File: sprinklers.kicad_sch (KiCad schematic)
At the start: 43 parts, among them J1 Conn_01x02, J2 Conn_01x02, J3 Conn_01x02, J4 Conn_01x02, J5 Conn_01x02, J6 Conn_01x02, K1 SANYOU_SRD_Form_C, K2 SANYOU_SRD_Form_C, K3 SANYOU_SRD_Form_C, K4 SANYOU_SRD_Form_C, K5 SANYOU_SRD_Form_C, K6 SANYOU_SRD_Form_C, Q1 Q_NMOS_GDS, Q2 Q_NMOS_GDS, Q3 Q_NMOS_GDS, Q4 Q_NMOS_GDS, Q5 Q_NMOS_GDS, Q6 Q_NMOS_GDS, U1 LM2596S-5, U2 ESP32-WROOM-32D, U3 AP1117-33

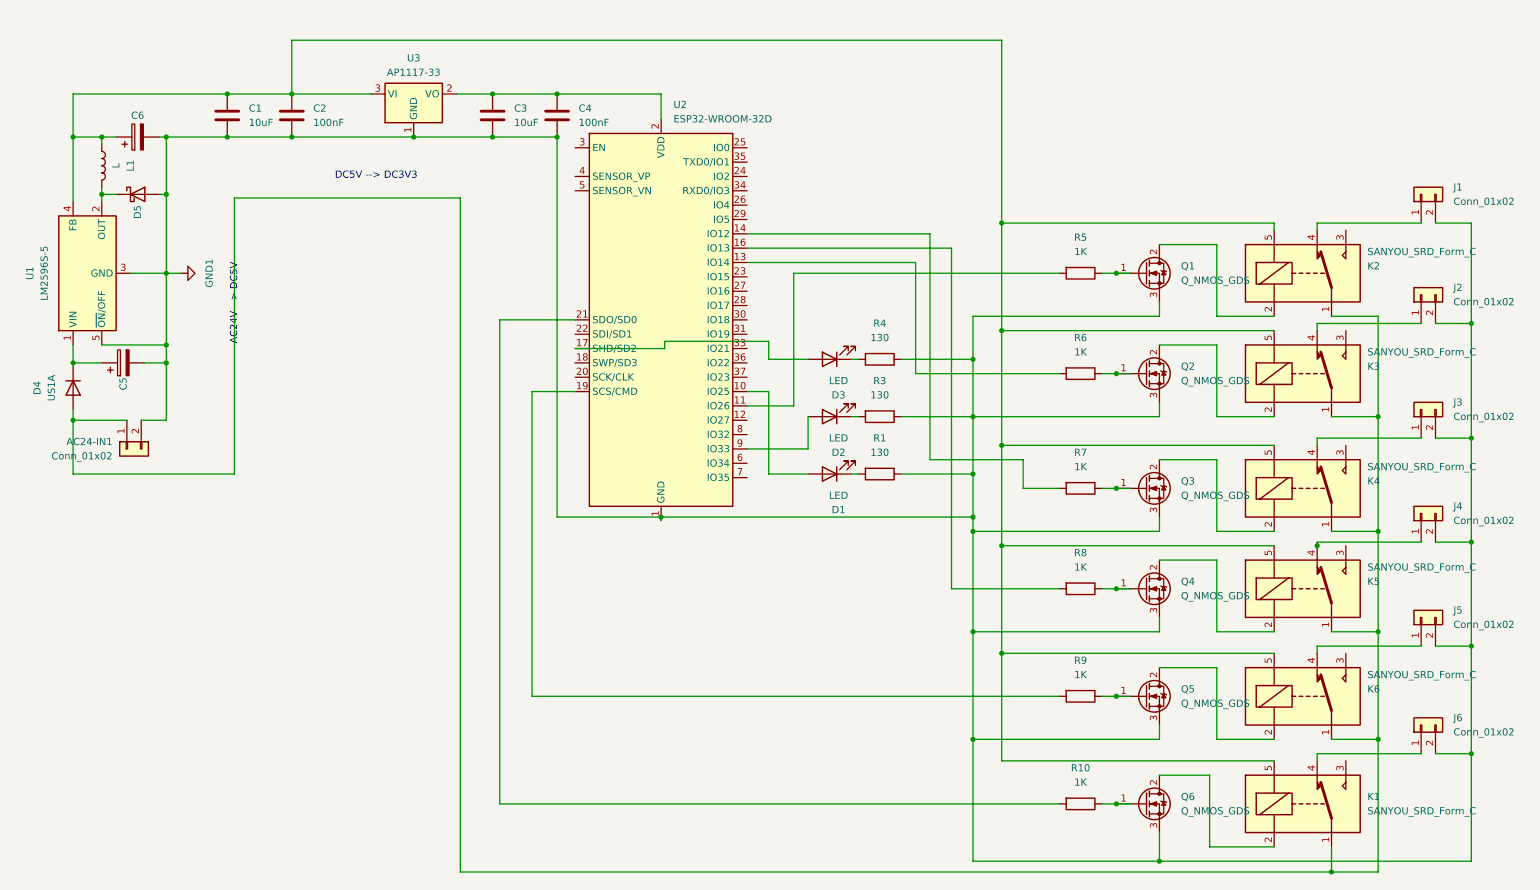
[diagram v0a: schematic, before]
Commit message: V1.1.0 with notation
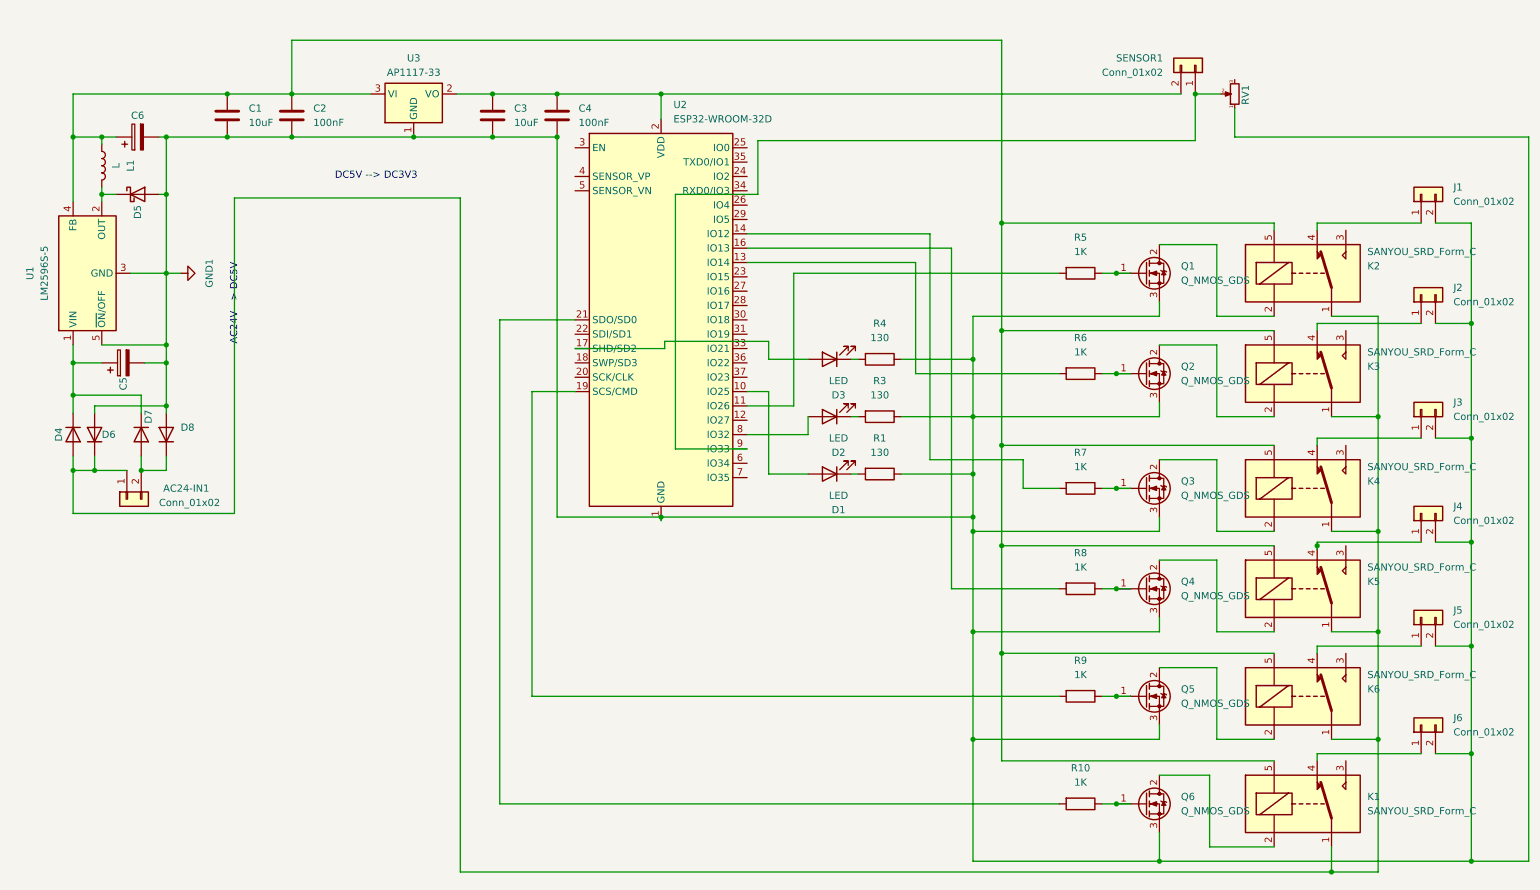
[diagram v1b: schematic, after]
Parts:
- added D6, D7, D8: 900mV@2A 30ns 2A 50V DO-214AA Diodes, Diode_SMD:D_SMB, symbol Diode:US1A
- added RV1: R_Potentiometer_Small, Potentiometer_THT:Potentiometer_Bourns_3296Y_Vertical, symbol Device:R_Potentiometer_Small
- added SENSOR1: Conn_01x02, Connector:JWT_A3963_1x02_P3.96mm_Vertical, symbol Connector_Generic:Conn_01x02
- AC24-IN1, J1, J2, J3, J4, J5, J6: LCSC C474894 -> C3031444
- C1: footprint Capacitor_SMD:C_0402_1005Metric -> Capacitor_SMD:C_0805_2012Metric
- C2, C4: footprint Capacitor_SMD:C_0402_1005Metric -> Capacitor_SMD:C_0603_1608Metric
- C3: footprint Capacitor_SMD:C_0402_1005Metric -> Capacitor_SMD:C_0805_2012Metric; LCSC C13585 -> C440198
- D1: LCSC C2297 -> C84256
- D2: LCSC C2296 -> C2297
- D3: LCSC C84256 -> C2296
- D4: value US1A -> 900mV@2A 30ns 2A 50V DO-214AA Diodes; footprint Diode_SMD:D_SMA -> Diode_SMD:D_SMB; LCSC C183422 -> C5224093
- Q1, Q2, Q3, Q4, Q5, Q6: LCSC C98152 -> C122491
- R9: LCSC C17451 -> C4410
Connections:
- net GND1: now also D6.2 (A), D8.2 (A), RV1.1; no longer AC24-IN1.2 (Pin_2)
- net at AC24-IN1.1 (Pin_1), D4.2 (A), K1.1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: now also D6.1 (K)
- net at C3.1, C4.1, U2.2 (VDD)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: now also SENSOR1.2 (Pin_2)
- net at C5.1, D4.1 (K), U1.1 (VIN): now also D7.1 (K)
- net at U2.9 (IO33): now also RV1.2, SENSOR1.1 (Pin_1); no longer D2.2 (A)
- net at U2.8 (IO32): now also D2.2 (A)
- new net: AC24-IN1.2 (Pin_2), D7.2 (A), D8.1 (K)
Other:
- moved on the sheet: AC24-IN1, D4

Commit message: applying fixed after review
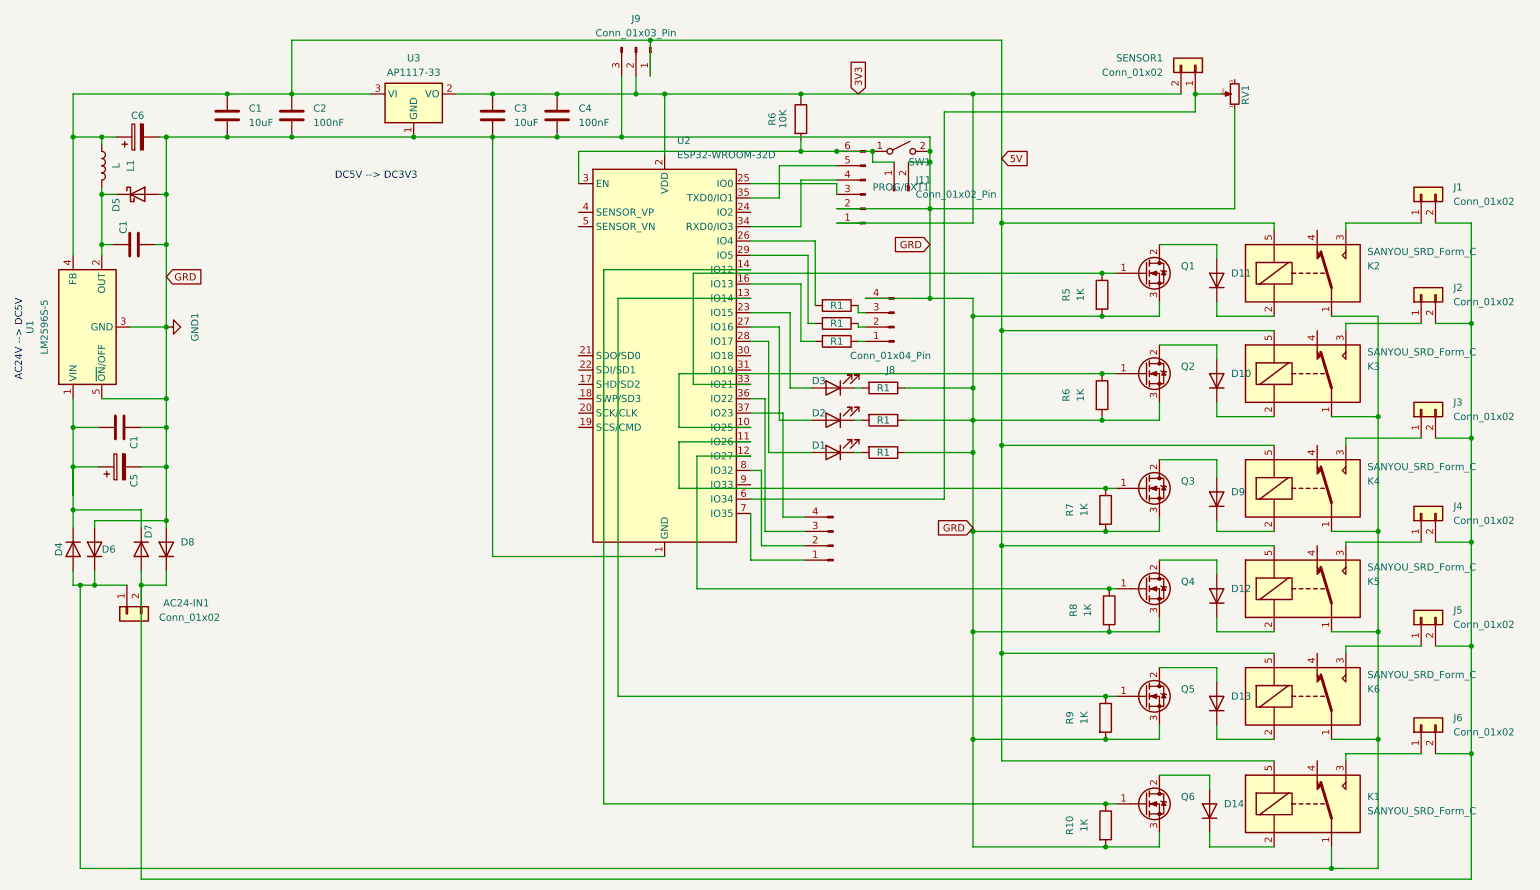
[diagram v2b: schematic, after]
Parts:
- removed R3, R4: 130, Resistor_SMD:R_1206_3216Metric, symbol Device:R
- removed R6: 1K, Resistor_SMD:R_1206_3216Metric, symbol Device:R
- added C1 (x2): 25V 1uF X5R ±10% 0402 Multilayer Ceramic Capacito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, Capacitor_SMD:C_01005_0402Metric, symbol Device:C
- added D10, D11, D12, D13, D14, D9: 75V 400mW Single 1V@50mA 4ns 150mA SOD-123 Switch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, Diode_SMD:D_SOD-123, symbol Diode:US1A
- added EXT1, J8: Conn_01x04_Pin, Connector_PinHeader_2.54mm:PinHeader_1x04_P2.54mm_Vertical, symbol Connector:Conn_01x04_Pin
- added J11: Conn_01x02_Pin, Connector_PinHeader_2.54mm:PinHeader_1x02_P2.54mm_Vertical, symbol Connector:Conn_01x02_Pin
- added J9: Conn_01x03_Pin, Connector_PinHeader_2.54mm:PinHeader_1x03_P2.54mm_Vertical, symbol Connector:Conn_01x03_Pin
- added PROG/EXT1: Conn_01x06_Pin, Connector_PinHeader_2.54mm:PinHeader_1x06_P2.54mm_Vertical, symbol Connector:Conn_01x06_Pin
- added R1 (x5): 130, Resistor_SMD:R_0201_0603Metric, symbol Device:R
- added R6: 10K, Resistor_SMD:R_1206_3216Metric, symbol Device:R
- added R6: 1K, Resistor_SMD:R_1206_3216Metric, symbol Device:R
- added SW1: SW_SPST, Button_Switch_SMD:SW_SPST_TL3342, symbol Switch:SW_SPST
- C5, C6: footprint Capacitor_THT:CP_Radial_D8.0mm_P3.50mm -> Capacitor_THT:CP_Radial_D10.0mm_P5.00mm; LCSC C225865 -> C461457
- D1: LCSC C84256 -> C130721
- D2: LCSC C2297 -> C130719
- D3: LCSC C2296 -> C130724
- K1, K2, K3, K4, K5, K6: LCSC C24585 -> C35449
- L1: LCSC C2983075 -> C339951
- Q1, Q2, Q3, Q4, Q5, Q6: LCSC C122491 -> C3010
- R1: footprint Resistor_SMD:R_1206_3216Metric -> Resistor_SMD:R_0201_0603Metric; LCSC C4410 -> C22797
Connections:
- net GND1: now also R10.2, R5.2, R7.2, R8.2, R9.2, C1.1, C1.1, J11.2 (Pin_2), J8.4 (Pin_4), J9.3 (Pin_3), PROG/EXT1.2 (Pin_2), R1.1, R1.1, R6.2, SW1.2 (B); no longer J1.2 (Pin_2), J2.2 (Pin_2), J3.2 (Pin_2), J4.2 (Pin_2), J5.2 (Pin_2), J6.2 (Pin_2)
- net at J3.1 (Pin_1): now also K4.3; no longer K4.4
- net at K1.2: now also D14.1 (K); no longer Q6.2 (D)
- net at K1.3: now also J6.1 (Pin_1)
- net at K1.4: no longer J6.1 (Pin_1)
- net 5V: now reaches C1.1, C2.1, C6.1, K1.5, K2.5, K3.5, K4.5, K5.5, K6.5, L1.2, U1.4 (FB), U3.3 (VI)
- net 5V: now also J9.1 (Pin_1)
- net at Q1.1 (G), R5.1: now also U2.33 (IO21)
- net at U2.11 (IO26): now also Q3.1 (G), R7.1; no longer R5.2
- net at J5.1 (Pin_1): now also K6.3; no longer K6.4
- net at D1.2 (A): now also U2.28 (IO17); no longer U2.10 (IO25)
- net at U2.14 (IO12): now also Q6.1 (G), R10.1; no longer R7.2
- net at J1.1 (Pin_1): now also K2.3; no longer K2.4
- net at K2.2: now also D11.1 (K); no longer Q1.2 (D)
- net at Q4.1 (G), R8.1: now also U2.12 (IO27)
- net at K5.2: now also D12.1 (K); no longer Q4.2 (D)
- net at C5.1, D4.1 (K), D7.1 (K)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: now also C1.2
- net at AC24-IN1.2 (Pin_2), D7.2 (A), D8.1 (K): now also J1.2 (Pin_2), J2.2 (Pin_2), J3.2 (Pin_2), J4.2 (Pin_2), J5.2 (Pin_2), J6.2 (Pin_2)
- net at D5.1 (K), L1.1, U1.2 (OUT): now also C1.2
- net at Q2.1 (G): now also U2.10 (IO25), R6.1
- net at Q2.2 (D): now also D10.2 (A); no longer K3.2
- net at U2.21 (SDO/SD0): no longer R10.2
- net at RV1.2, SENSOR1.1 (Pin_1): now also U2.6 (IO34); no longer U2.9 (IO33)
- net 3V3: now reaches C3.1, C4.1, SENSOR1.2 (Pin_2), U2.2 (VDD), U3.2 (VO)
- net 3V3: now also J9.2 (Pin_2), PROG/EXT1.1 (Pin_1), R6.1
- net at K4.2: now also D9.1 (K); no longer Q3.2 (D)
- net at K5.3: now also J4.1 (Pin_1)
- net at K5.4: no longer J4.1 (Pin_1)
- net at D3.1 (K): now also R1.2
- net at D2.1 (K): now also R1.2
- net at D3.2 (A): now also U2.23 (IO15); no longer U2.17 (SHD/SD2)
- net at K6.2: now also D13.1 (K); no longer Q5.2 (D)
- net at J2.1 (Pin_1): now also K3.3; no longer K3.4
- net at Q5.1 (G), R9.1: now also U2.13 (IO14)
- net at U2.19 (SCS/CMD): no longer R9.2
- net at U2.8 (IO32): now also EXT1.2 (Pin_2); no longer D2.2 (A)
- net at U2.16 (IO13): now also R1.2; no longer R8.2
- net at U2.25 (IO0): now also PROG/EXT1.3 (Pin_3)
- net at U2.26 (IO4): now also R1.2
- net at U2.27 (IO16): now also D2.2 (A)
- net at U2.29 (IO5): now also R1.2
- net at U2.3 (EN): now also J11.1 (Pin_1), PROG/EXT1.6 (Pin_6), R6.2, SW1.1 (A)
- net at U2.34 (RXD0/IO3): now also PROG/EXT1.4 (Pin_4)
- net at U2.35 (TXD0/IO1): now also PROG/EXT1.5 (Pin_5)
- net at U2.36 (IO22): now also EXT1.3 (Pin_3)
- net at U2.37 (IO23): now also EXT1.4 (Pin_4)
- net at U2.7 (IO35): now also EXT1.1 (Pin_1)
- new net: D11.2 (A), Q1.2 (D)
- new net: J8.2 (Pin_2), R1.1
- new net: D13.2 (A), Q5.2 (D)
- new net: D12.2 (A), Q4.2 (D)
- new net: J8.1 (Pin_1), R1.1
- new net: D14.2 (A), Q6.2 (D)
- new net: D10.1 (K), K3.2
- new net: D9.2 (A), Q3.2 (D)
- new net: J8.3 (Pin_3), R1.1
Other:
- moved on the sheet: AC24-IN1, C5, D1, D2, D3, D4, D6, D7, D8, R1, U1, U2
